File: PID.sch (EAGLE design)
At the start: 32 parts, among them IC1 UA741CPE4, IC2 UA741CPE4, IC3 UA741CPE4, IC4 UA741CPE4, IC5 UA741CPE4

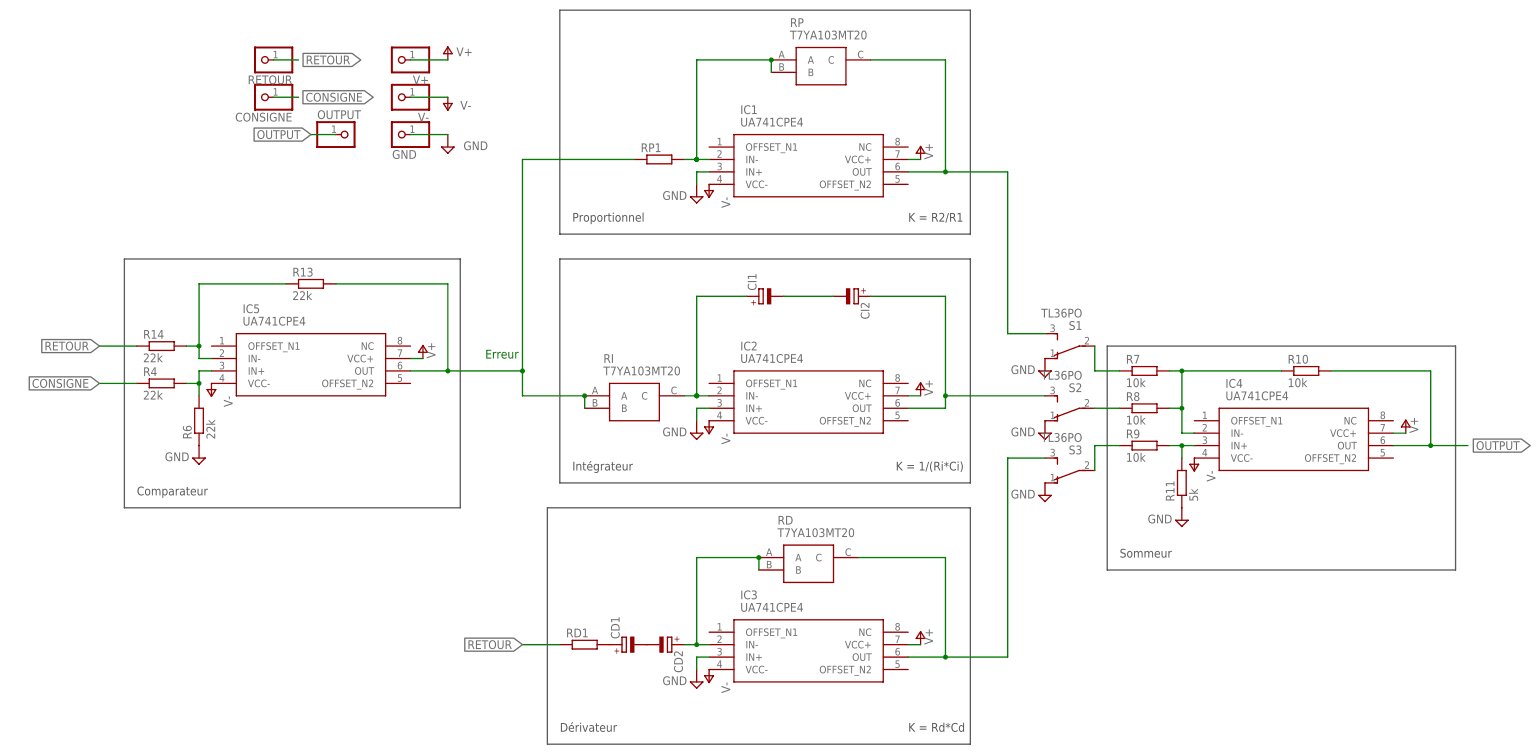
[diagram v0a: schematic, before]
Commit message: couocu
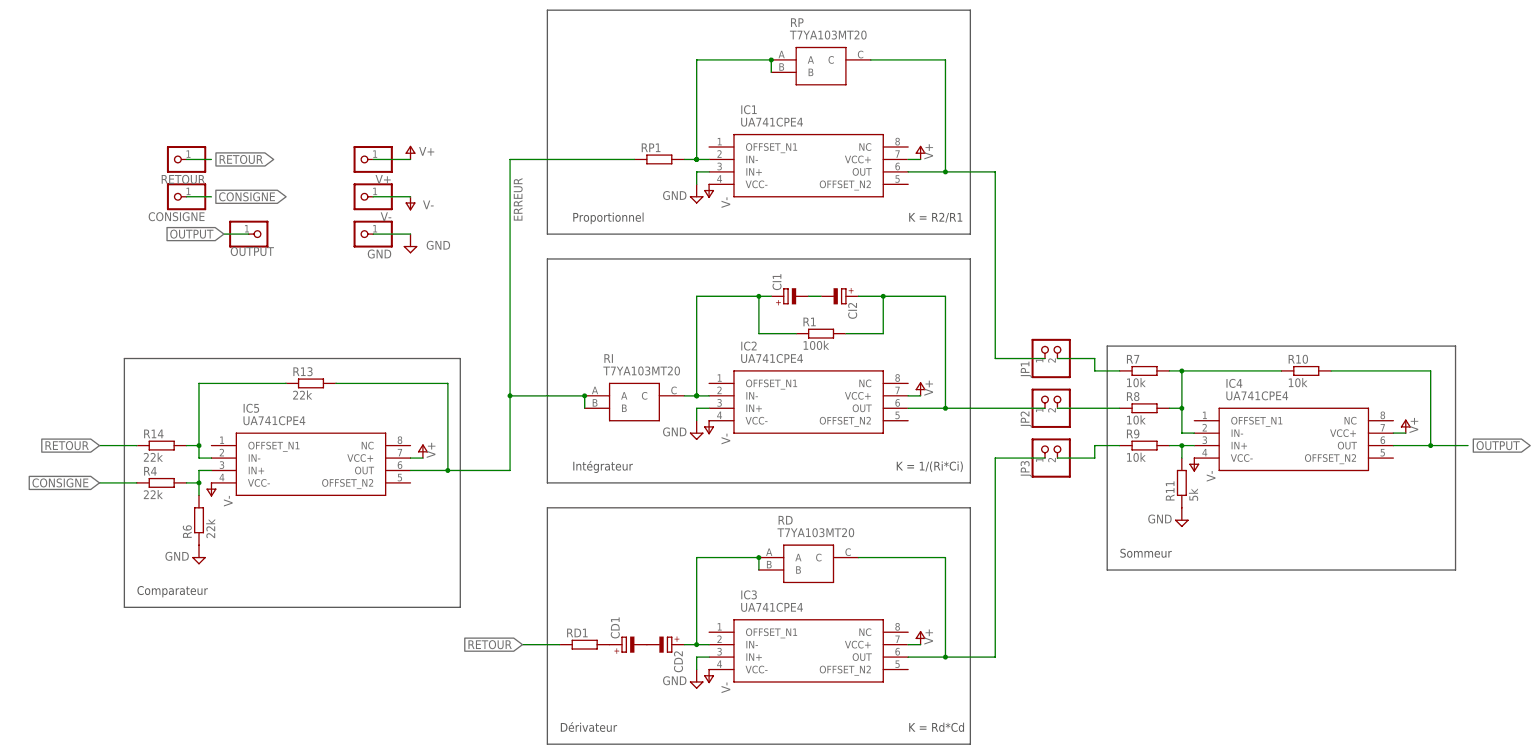
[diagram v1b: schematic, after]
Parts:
- removed S1, S2, S3: TL36PO, switch:TL36PO
- added JP1, JP2, JP3: (no value), pinhead:PINHD-1X2
- added R1: 100k, rcl:R-EU_0204/7
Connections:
- net N$15 renamed ERREUR
- net GND: no longer S1.O, S2.O, S3.O
- net N$10: now also JP3.1; no longer S3.S
- net N$12: now also JP1.2; no longer S1.P
- net N$16: now also JP2.2; no longer S2.P
- net N$19: now also JP3.2; no longer S3.P
- net N$2: now also JP1.1; no longer S1.S
- net N$4: now also JP2.1, R1.2; no longer S2.S
- net N$5: now also R1.1
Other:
- note removed: "Erreur"
- moved on the sheet: CI1, CI2, CONSIGNE, GND, IC5, OUTPUT, R13, R14, R4, R6, RETOUR, V+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
